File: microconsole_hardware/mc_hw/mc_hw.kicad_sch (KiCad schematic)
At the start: 10 parts

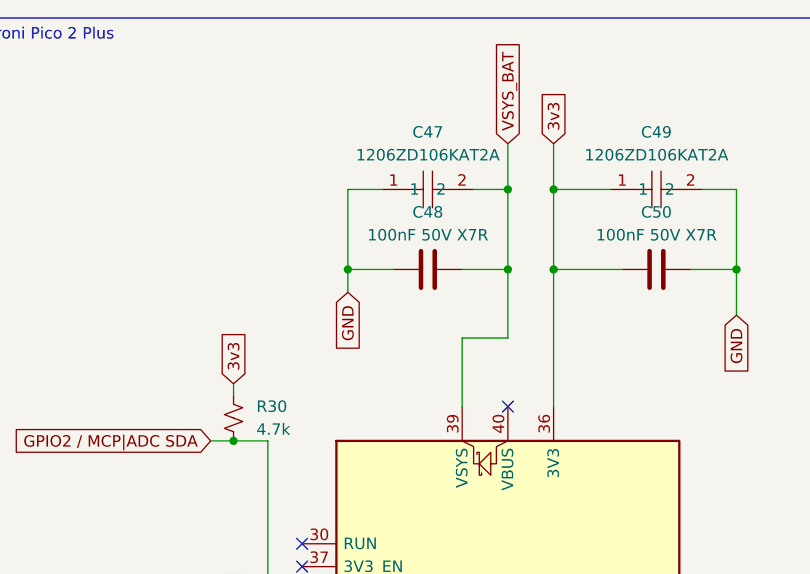
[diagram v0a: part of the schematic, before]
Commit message: fixup
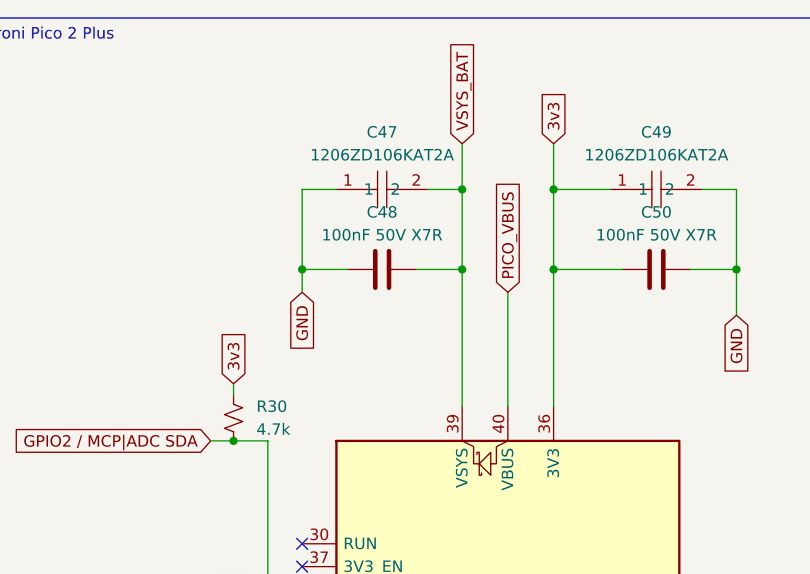
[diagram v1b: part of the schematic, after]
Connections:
- net PICO_VBUS: now reaches A2.40 (VBUS)
- no-connect marks 19 -> 18
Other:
- moved on the sheet: C47, C48
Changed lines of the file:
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@@
 	)
 	(junction
-		(at 204.47 54.61)
+		(at 199.39 54.61)
 		(diameter 0)
 		(color 0 0 0 0)
 	)
 	(junction
-		(at 204.47 63.5)
+		(at 199.39 63.5)
 		(diameter 0)
 		(color 0 0 0 0)
@@
 	)
 	(junction
-		(at 186.69 63.5)
+		(at 181.61 63.5)
 		(diameter 0)
 		(color 0 0 0 0)
@@
 	)
 	(no_connect
-		(at 204.47 78.74)
-	)
-	(no_connect
 		(at 227.33 139.7)
 	)
@@
 	(wire
 		(pts
-			(xy 190.5 54.61) (xy 186.69 54.61)
+			(xy 185.42 54.61) (xy 181.61 54.61)
 		)
 		(stroke
@@
 	(wire
 		(pts
-			(xy 186.69 54.61) (xy 186.69 63.5)
+			(xy 181.61 54.61) (xy 181.61 63.5)
 		)
 		(stroke
@@
 	(wire
 		(pts
+			(xy 204.47 66.04) (xy 204.47 78.74)
+		)
+		(stroke
+			(width 0)
+			(type default)
+		)
+	)
+	(wire
+		(pts
 			(xy 173.99 76.2) (xy 173.99 77.47)
 		)
@@
 	(wire
 		(pts
-			(xy 204.47 49.53) (xy 204.47 54.61)
+			(xy 199.39 49.53) (xy 199.39 54.61)
 		)
 		(stroke
@@
 	(wire
 		(pts
-			(xy 204.47 54.61) (xy 204.47 63.5)
+			(xy 199.39 54.61) (xy 199.39 63.5)
 		)
 		(stroke
@@
 	(wire
 		(pts
-			(xy 200.66 54.61) (xy 204.47 54.61)
+			(xy 195.58 54.61) (xy 199.39 54.61)
 		)
 		(stroke
@@
 	(wire
 		(pts
-			(xy 186.69 63.5) (xy 191.77 63.5)
+			(xy 181.61 63.5) (xy 186.69 63.5)
 		)
 		(stroke
@@
 	(wire
 		(pts
-			(xy 186.69 63.5) (xy 186.69 66.04)
-		)
-		(stroke
-			(width 0)
-			(type default)
-		)
-	)
-	(wire
-		(pts
-			(xy 199.39 71.12) (xy 204.47 71.12)
-		)
-		(stroke
-			(width 0)
-			(type default)
-		)
-	)
-	(wire
-		(pts
-			(xy 199.39 71.12) (xy 199.39 78.74)
+			(xy 181.61 63.5) (xy 181.61 66.04)
 		)
 		(stroke
@@
 	(wire
 		(pts
-			(xy 199.39 63.5) (xy 204.47 63.5)
+			(xy 194.31 63.5) (xy 199.39 63.5)
 		)
 		(stroke
@@
 	(wire
 		(pts
-			(xy 204.47 71.12) (xy 204.47 63.5)
+			(xy 199.39 63.5) (xy 199.39 78.74)
 		)
 		(stroke
@@
 		)
 	)
+	(global_label "PICO_VBUS"
+		(shape input)
+		(at 204.47 66.04 90)
+		(fields_autoplaced yes)
+		(effects
+			(font
+				(size 1.27 1.27)
+			)
+			(justify left)
+		)
+		(property "Intersheetrefs" "${INTERSHEET_REFS}"
+			(at 204.47 52.7133 90)
+			(hide yes)
+			(show_name no)
+			(do_not_autoplace no)
+			(effects
+				(font
+					(size 1.27 1.27)
+				)
+				(justify left)
+			)
+		)
+	)
 	(global_label "GPIO20 {slash} MAX DIN"
 		(shape input)
@@
 	(global_label "VSYS_BAT"
 		(shape input)
-		(at 204.47 49.53 90)
+		(at 199.39 49.53 90)
 		(fields_autoplaced yes)
 		(effects
@@
 		)
 		(property "Intersheetrefs" "${INTERSHEET_REFS}"
-			(at 204.47 37.6548 90)
+			(at 199.39 37.6548 90)
 			(hide yes)
 			(show_name no)
@@
 	(global_label "GND"
 		(shape input)
-		(at 186.69 66.04 270)
+		(at 181.61 66.04 270)
 		(fields_autoplaced yes)
 		(effects
@@
 		)
 		(property "Intersheetrefs" "${INTERSHEET_REFS}"
-			(at 186.69 72.8957 90)
+			(at 181.61 72.8957 90)
 			(hide yes)
 			(show_name no)
@@
 	(symbol
 		(lib_id "project_parts:C0805C104K5RAC7210")
-		(at 195.58 63.5 90)
+		(at 190.5 63.5 90)
 		(unit 1)
 		(body_style 1)
@@
 		(fields_autoplaced yes)
 		(property "Reference" "C48"
-			(at 195.58 57.15 90)
+			(at 190.5 57.15 90)
 			(show_name no)
 			(do_not_autoplace no)
@@
 		)
 		(property "Value" "100nF 50V X7R"
-			(at 195.58 59.69 90)
+			(at 190.5 59.69 90)
 			(show_name no)
 			(do_not_autoplace no)
@@
 		)
 		(property "Footprint" "project_parts:C_0805_2012Metric_KEMET_IPC-B"
-			(at 195.58 63.5 0)
+			(at 190.5 63.5 0)
 			(hide yes)
 			(show_name no)
@@
 		)
 		(property "Datasheet" ""
-			(at 195.58 63.5 0)
+			(at 190.5 63.5 0)
 			(hide yes)
 			(show_name no)
@@
 		)
 		(property "Description" "KEMET 0805 MLCC 0.1uF 10% 50V X7R"
-			(at 195.58 63.5 0)
+			(at 190.5 63.5 0)
 			(hide yes)
 			(show_name no)
@@
 		)
 		(property "MPN" "C0805C104K5RAC7210"
-			(at 195.58 63.5 0)
+			(at 190.5 63.5 0)
 			(hide yes)
 			(show_name no)
@@
 		)
 		(property "Manufacturer" "KEMET"
-			(at 195.58 63.5 0)
+			(at 190.5 63.5 0)
 			(hide yes)
 			(show_name no)
@@
 	(symbol
 		(lib_id "project_parts:1206ZD106KAT2A")
-		(at 195.58 54.61 0)
+		(at 190.5 54.61 0)
 		(unit 1)
 		(body_style 1)
@@
 		(fields_autoplaced yes)
 		(property "Reference" "C47"
-			(at 195.58 48.26 0)
+			(at 190.5 48.26 0)
 			(show_name no)
 			(do_not_autoplace no)
@@
 		)
 		(property "Value" "1206ZD106KAT2A"
-			(at 195.58 50.8 0)
+			(at 190.5 50.8 0)
 			(show_name no)
 			(do_not_autoplace no)
@@
 		)
 		(property "Footprint" "project_parts:C1206"
-			(at 195.58 62.23 0)
+			(at 190.5 62.23 0)
 			(hide yes)
 			(show_name no)
@@
 		)
 		(property "Datasheet" "https://lcsc.com/product-detail/presales_AVX-1206ZD106KAT2A_C597553.html"
-			(at 195.58 64.77 0)
+			(at 190.5 64.77 0)
 			(hide yes)
 			(show_name no)
@@
 		)
 		(property "Description" ""
-			(at 195.58 54.61 0)
+			(at 190.5 54.61 0)
 			(hide yes)
 			(show_name no)
@@
 		)
 		(property "Manufacturer" "Kyocera AVX"
-			(at 195.58 67.31 0)
+			(at 190.5 67.31 0)
 			(hide yes)
 			(show_name no)
@@
 		)
 		(property "MPN" "1206ZD106KAT2A"
-			(at 195.58 69.85 0)
+			(at 190.5 69.85 0)
 			(hide yes)
 			(show_name no)
@@
 		)
 		(property "LCSC Part" "C597553"
-			(at 195.58 72.39 0)
-			(hide yes)
-			(show_name no)
+			(at 190.5 72.39 0)
+			(hide yes)
+			(show_name no)
